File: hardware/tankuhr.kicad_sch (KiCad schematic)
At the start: 33 parts, among them J1 Conn_01x04_Pin, J2 Conn_01x04_Pin, J3 Conn_01x04_Pin, U1 TBA1-1211, U2 XIAO-ESP32-C3-SMD

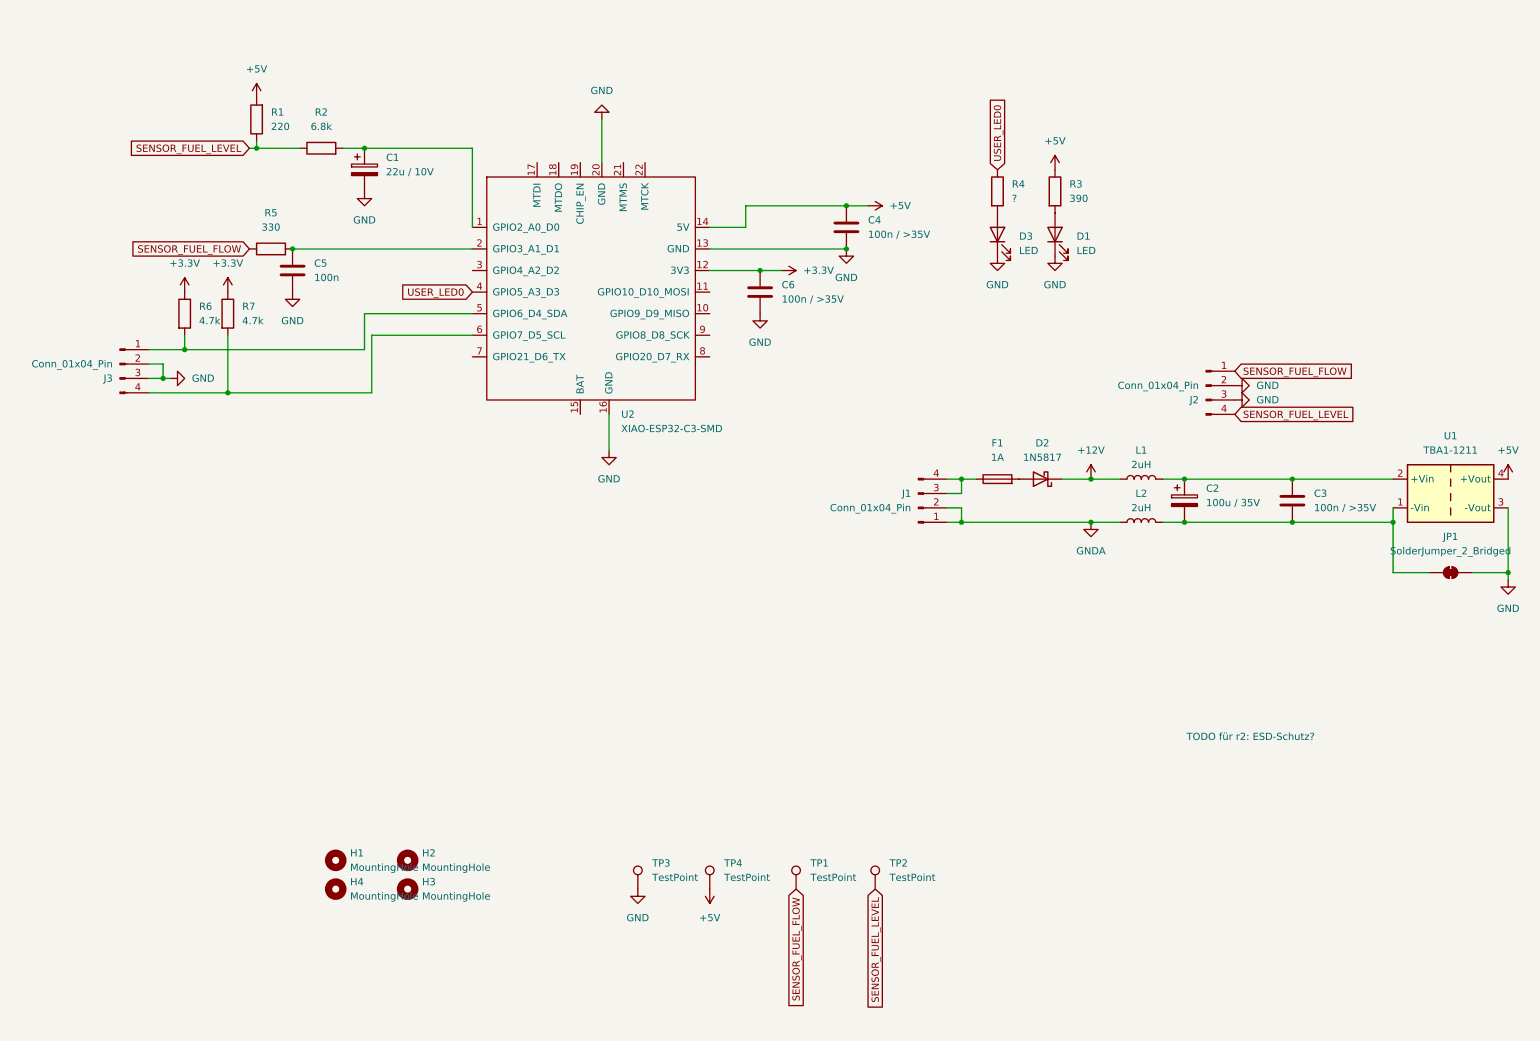
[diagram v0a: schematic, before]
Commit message: WIP
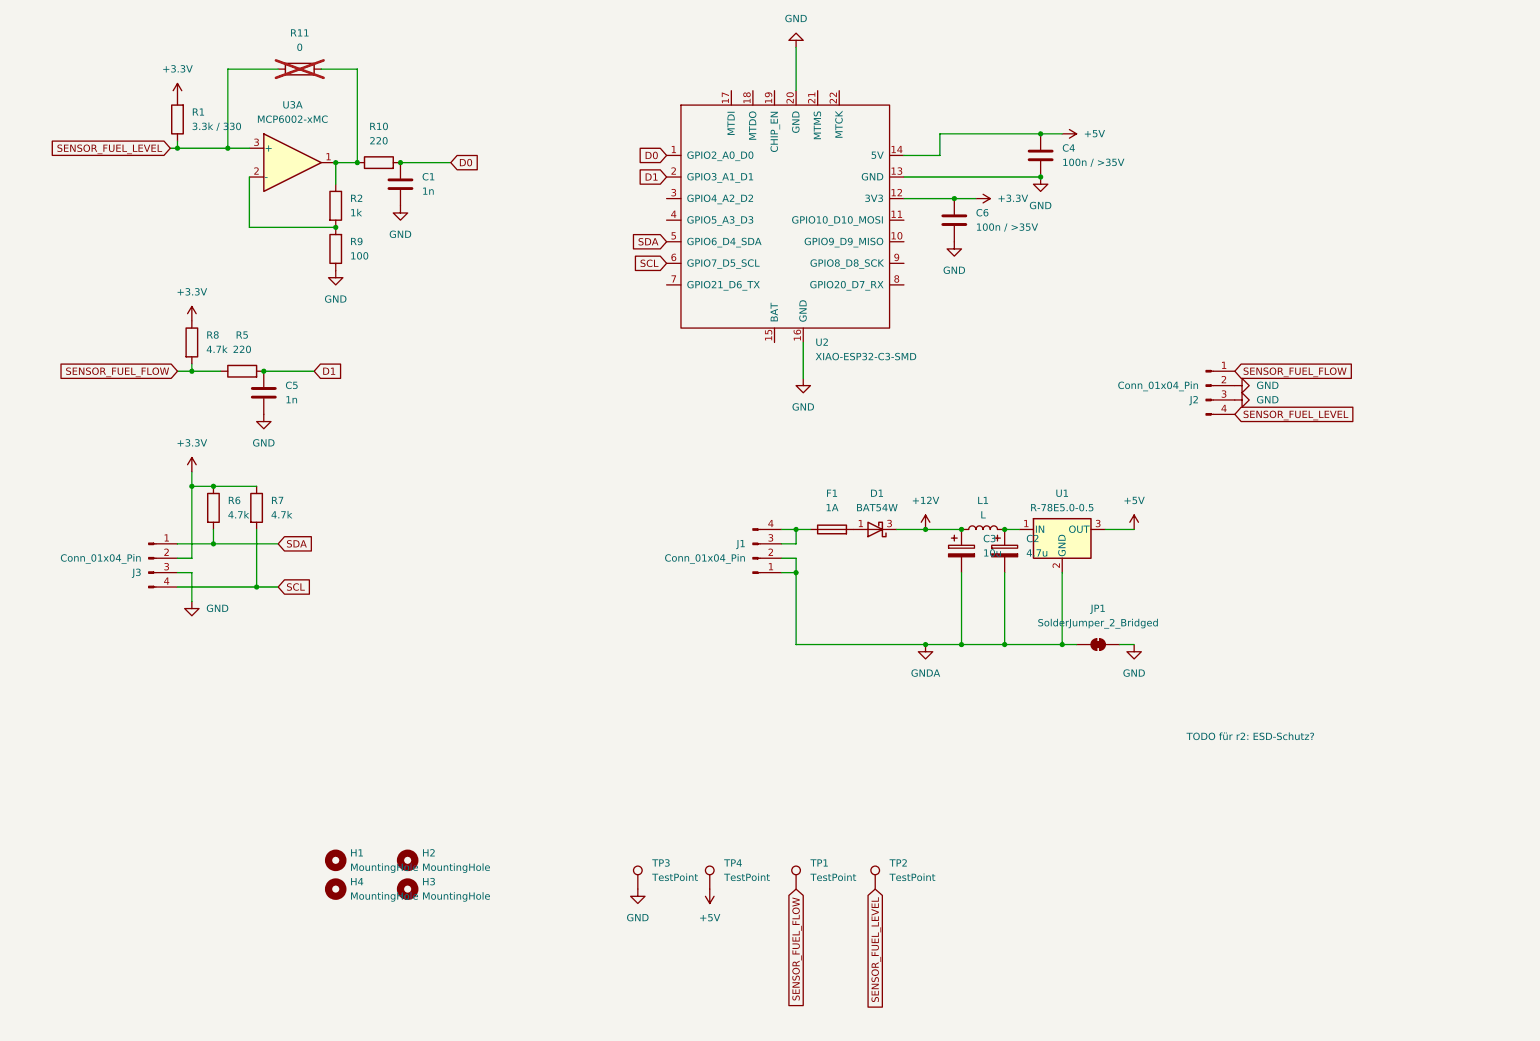
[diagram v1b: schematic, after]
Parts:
- removed C1: 22u / 10V, Capacitor_THT:CP_Radial_D4.0mm_P1.50mm, symbol Device:C_Polarized
- removed C3: 100n / >35V, Capacitor_SMD:C_0805_2012Metric_Pad1.18x1.45mm_HandSolder, symbol Device:C
- removed D1, D3: LED, LED_SMD:LED_PLCC-2_3.4x3.0mm_AK, symbol Device:LED
- removed D2: 1N5817, Diode_THT:D_DO-41_SOD81_P7.62mm_Horizontal, symbol Device:D_Schottky
- removed L2: 2uH, Inductor_THT:L_Axial_L7.0mm_D3.3mm_P10.16mm_Horizontal_Fastron_MICC, symbol Device:L
- removed R3: 390, Resistor_SMD:R_0805_2012Metric_Pad1.20x1.40mm_HandSolder, symbol Device:R
- removed R4: ?, Resistor_SMD:R_0805_2012Metric_Pad1.20x1.40mm_HandSolder, symbol Device:R
- removed U1: TBA1-1211, Converter_DCDC:Converter_DCDC_TRACO_TBA1-xxxx_THT, symbol Converter_DCDC:TBA1-1211
- added C1: 1n, Capacitor_SMD:C_0805_2012Metric_Pad1.18x1.45mm_HandSolder, symbol Device:C
- added C3: 10u, Capacitor_THT:CP_Radial_D5.0mm_P2.00mm, symbol Device:C_Polarized
- added D1: BAT54W, Package_TO_SOT_SMD:SOT-323_SC-70, symbol Diode:BAT54W
- added R10: 220, Resistor_SMD:R_0805_2012Metric_Pad1.20x1.40mm_HandSolder, symbol Device:R
- added R11: 0, Resistor_SMD:R_0805_2012Metric_Pad1.20x1.40mm_HandSolder, symbol Device:R
- added R8: 4.7k, Resistor_SMD:R_0805_2012Metric_Pad1.20x1.40mm_HandSolder, symbol Device:R
- added R9: 100, Resistor_SMD:R_0805_2012Metric_Pad1.20x1.40mm_HandSolder, symbol Device:R
- added U1: R-78E5.0-0.5, Converter_DCDC:Converter_DCDC_RECOM_R-78E-0.5_THT, symbol Regulator_Switching:R-78E5.0-0.5
- added U3: MCP6002-xMC, Package_DFN_QFN:DFN-8-1EP_3x2mm_P0.5mm_EP1.75x1.45mm, symbol Amplifier_Operational:MCP6002-xMC
- C2: value 100u / 35V -> 4.7u; footprint Capacitor_THT:CP_Radial_D8.0mm_P3.50mm -> Capacitor_THT:CP_Radial_D5.0mm_P2.00mm
- C5: value 100n -> 1n
- L1: value 2uH -> L; footprint Inductor_THT:L_Axial_L7.0mm_D3.3mm_P10.16mm_Horizontal_Fastron_MICC -> asdf:RECOM RLS-126
- R1: value 220 -> 3.3k / 330
- R2: value 6.8k -> 1k
- R5: value 330 -> 220
- R6, R7: footprint Capacitor_SMD:C_0805_2012Metric_Pad1.18x1.45mm_HandSolder -> Resistor_SMD:R_0805_2012Metric_Pad1.20x1.40mm_HandSolder
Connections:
- net +12V: now also C3.1, D1.3 (K)
- net +3.3V: now also J3.2 (Pin_2), R1.2, R8.1
- net +5V: now also U1.3 (OUT); no longer R1.2
- net GND: now also C1.2, R9.1; no longer J3.2 (Pin_2)
- net GNDA: now also C2.2, JP1.1 (A), C3.2, U1.2 (GND)
- net SENSOR_FUEL_FLOW: now also R8.2
- net SENSOR_FUEL_LEVEL: now also R11.1, U3.3 (+); no longer R2.1
- net at C2.1, L1.2: now also U1.1 (IN)
- net SDA: now reaches J3.1 (Pin_1), R6.2, U2.5 (GPIO6_D4_SDA)
- net at R2.2: now also R9.2, U3.2 (-); no longer U2.1 (GPIO2_A0_D0)
- net D1: now reaches C5.1, R5.2, U2.2 (GPIO3_A1_D1)
- net SCL: now reaches J3.4 (Pin_4), R7.2, U2.6 (GPIO7_D5_SCL)
- net at F1.2: now also D1.1 (A)
- net USER_LED0: no longer names the net of U2.4 (GPIO5_A3_D3)
- new net: R10.1, R11.2, R2.1, U3.1
- new net D0: C1.1, R10.2, U2.1 (GPIO2_A0_D0)
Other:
- moved on the sheet: C4, C5, C6, F1, J1, J3, JP1, R1, R5, R6, R7, U2
